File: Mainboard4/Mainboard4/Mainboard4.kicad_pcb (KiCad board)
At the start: 2 copper layers, 145.9 x 180.3 mm, 60 parts, among them J0 Conn_01x18, J1 Conn_01x18, J2 Conn_01x18, J3 Conn_01x18, J4 Conn_01x18, J5 Conn_01x18, J6_LEDS1 Conn_02x08_Odd_Even, J8 Conn_01x12_Female, U1 LM317_TO220, U2 STM32_F4xx, U3 LM317_TO220, U4 MCP2551-I-P, U5 ULN2803A, U6 ULN2803A, U7 ULN2803A

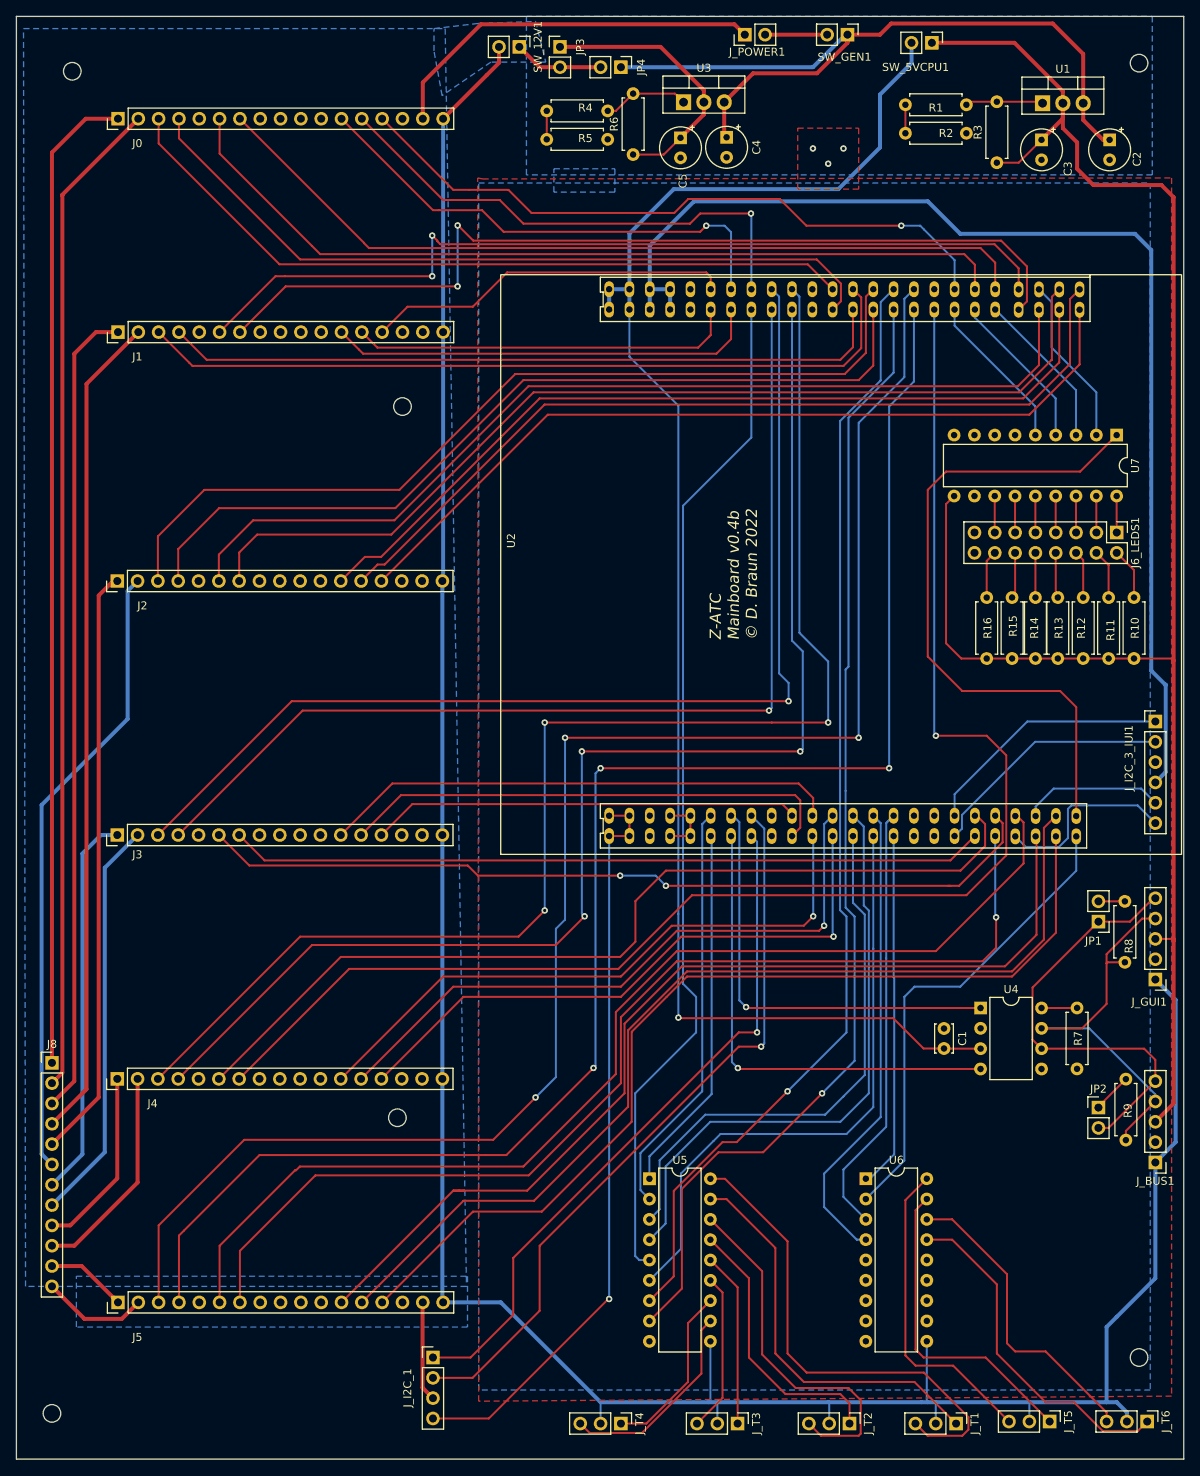
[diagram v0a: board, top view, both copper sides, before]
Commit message: ..
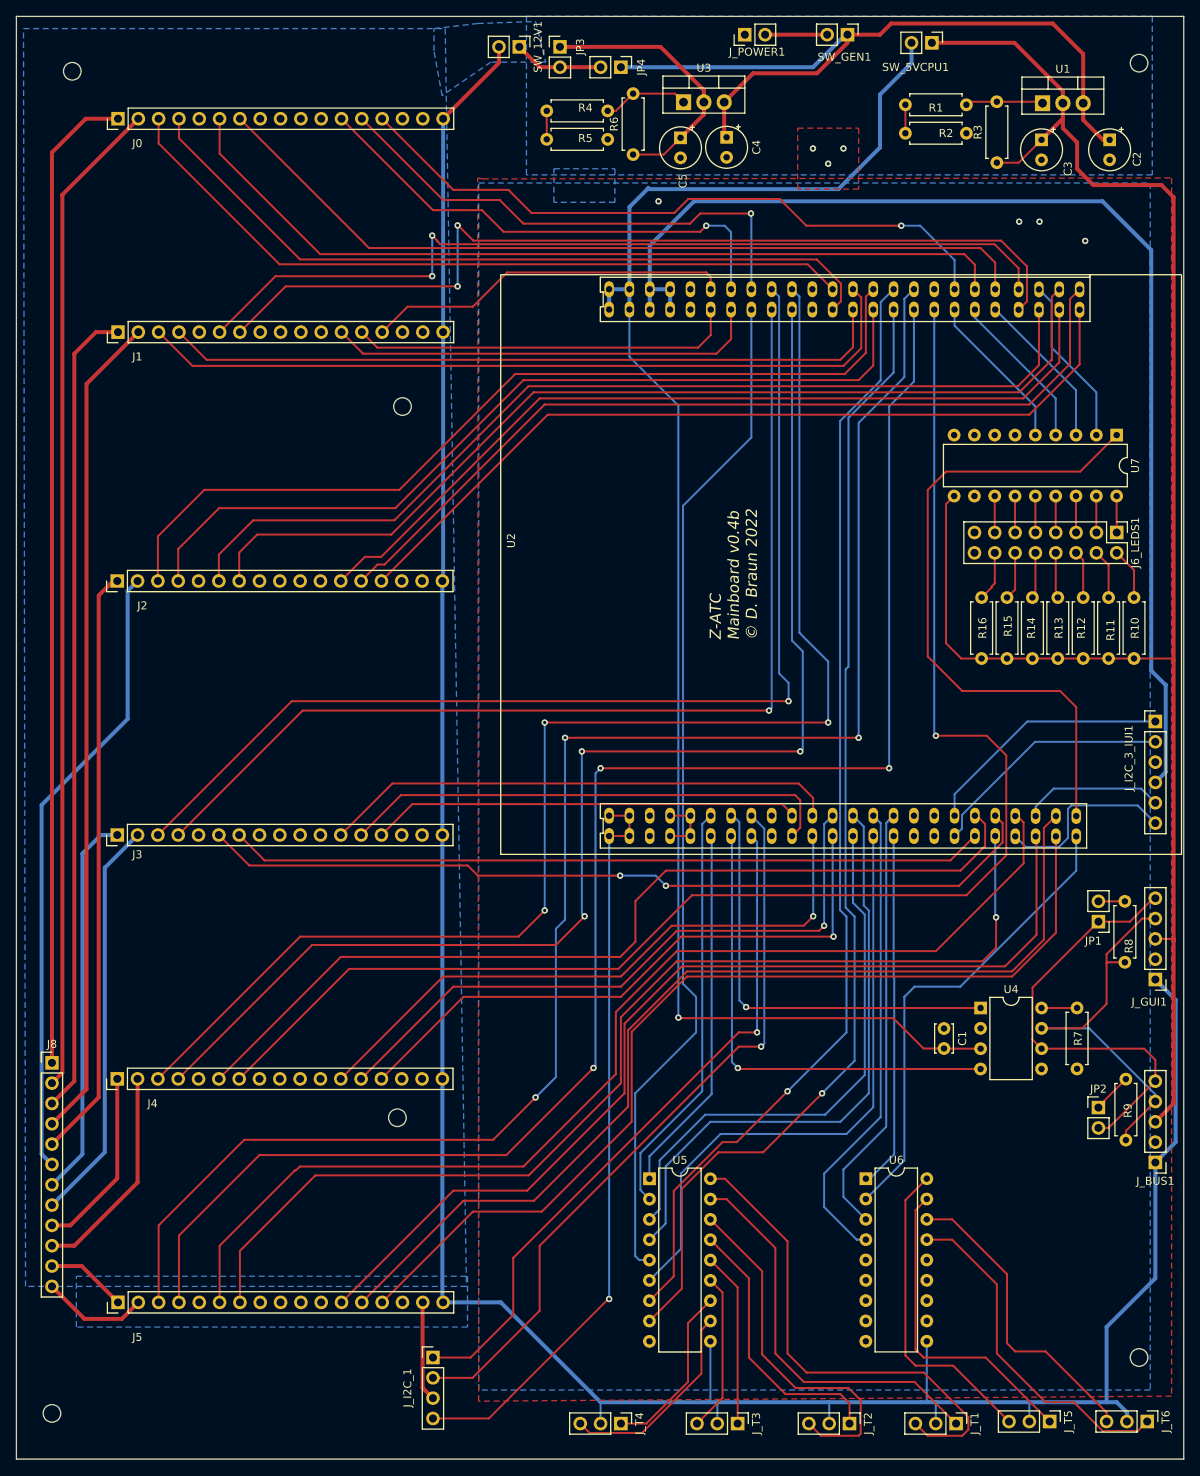
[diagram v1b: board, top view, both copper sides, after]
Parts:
- moved R16 0.64 mm to (156.3, 103.1)
- moved R15 0.63 mm to (159.5, 103.1)
- moved R14 0.38 mm to (162.7, 103.1)
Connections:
- net TURN4A renamed BOARD_LED
- net TURN4B renamed BOARD_LED2
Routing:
- net GND: track 68.5 -> 20.1 mm, vias 3 -> 7
- net 5VCPU: track 195.3 -> 197.3 mm
- net 5V: track 222.3 -> 220.4 mm
- net CT5_1: track 124.8 -> 123.4 mm
